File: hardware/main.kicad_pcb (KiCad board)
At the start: 2 copper layers, 50.5 x 28 mm, 40 parts, among them J1 2.54-1*5P, J2 KH-2.54FH-1X2P-H8.5, U1 74HC595, U2 74HC595

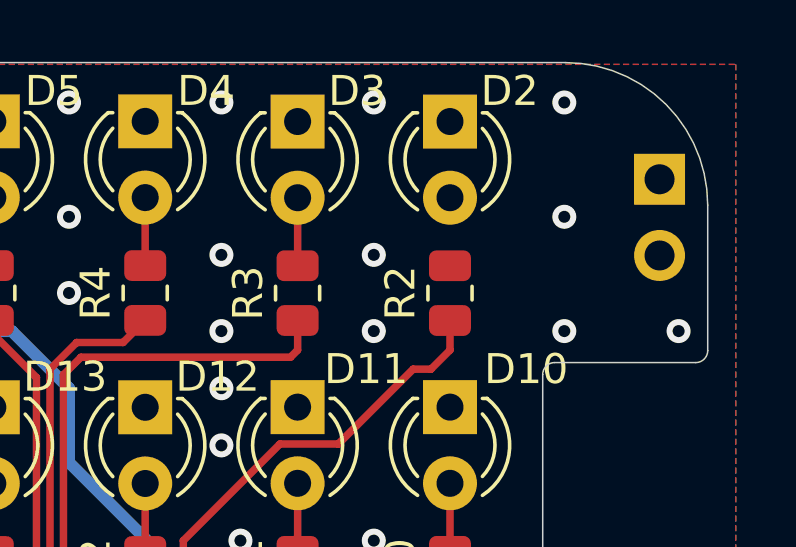
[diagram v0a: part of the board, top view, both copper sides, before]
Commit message: fix pcb
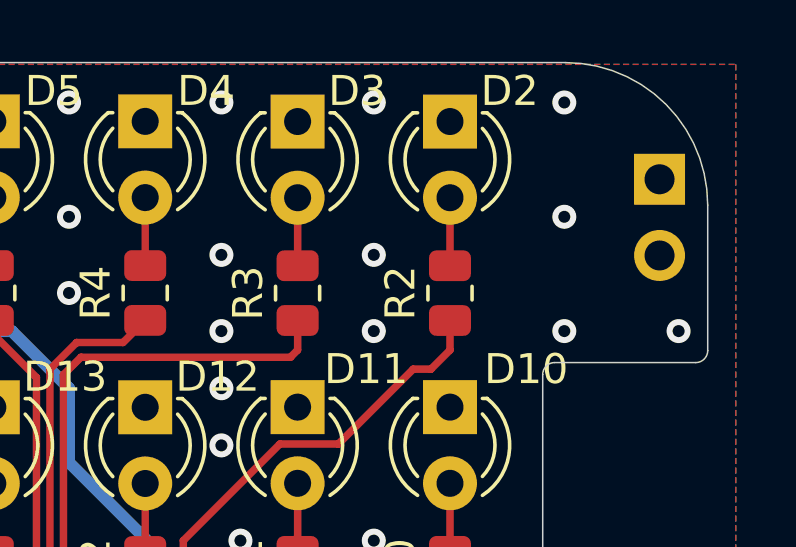
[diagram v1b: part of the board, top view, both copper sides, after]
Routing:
- net Net-(D2-A): track 0.00 -> 2.27 mm
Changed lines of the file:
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@@
+	)
+	(segment
+		(start 70.91 35.7725)
+		(end 70.91 33.505)
+		(width 0.25)
+		(layer "F.Cu")
+		(net 4)
 	)
 	(segment
